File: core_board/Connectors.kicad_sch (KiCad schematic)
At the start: 26 parts, among them J10 Conn_01x04_Pin, J11 Conn_01x04_Pin, J12 Conn_01x04_Pin, J14 Conn_01x04_Pin, J15 Conn_01x04_Pin, J3 Conn_01x04_Pin, J4 Conn_01x04_Pin, J5 Conn_01x04_Pin, J6 Conn_01x04_Pin, J7 Conn_01x02_Pin, J9 Conn_01x02_Pin, Q10 BSS138, Q11 BSS138, Q12 BSS138, Q13 BSS138, Q14 BSS138, Q9 BSS138

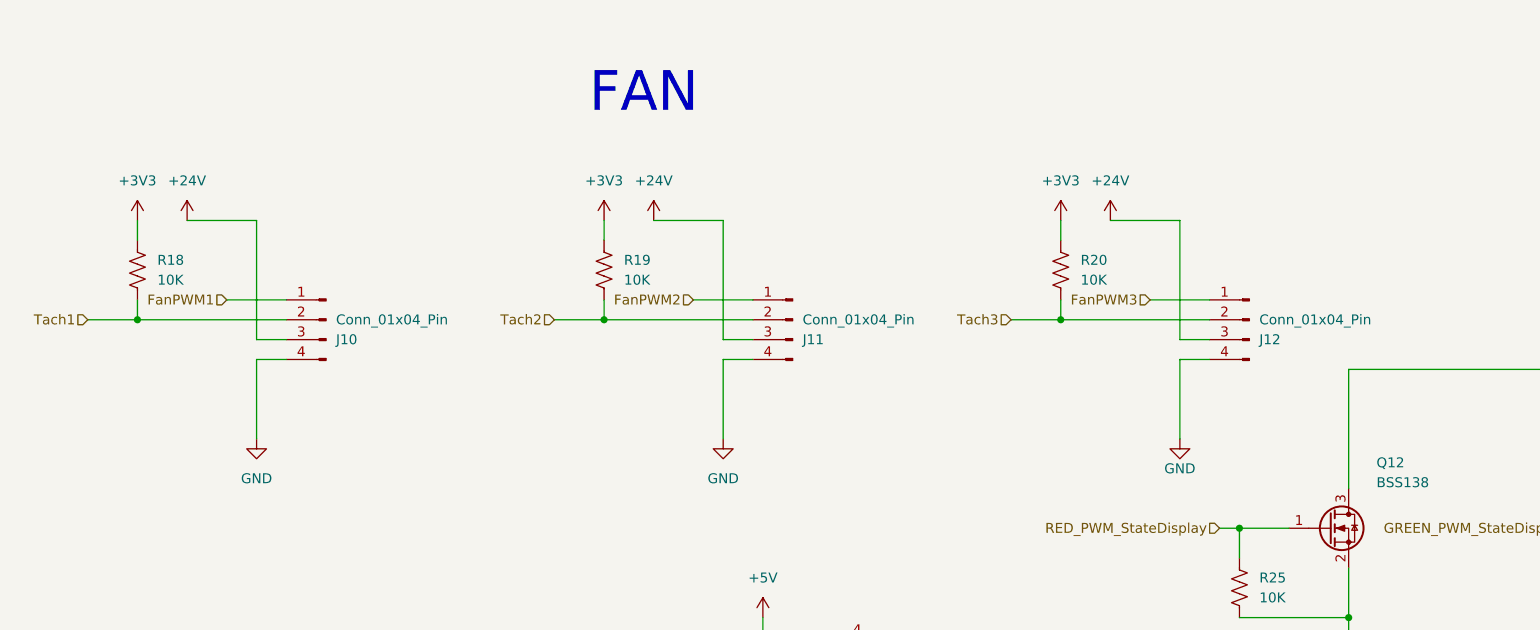
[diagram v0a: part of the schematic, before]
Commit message: Fix fan connectors
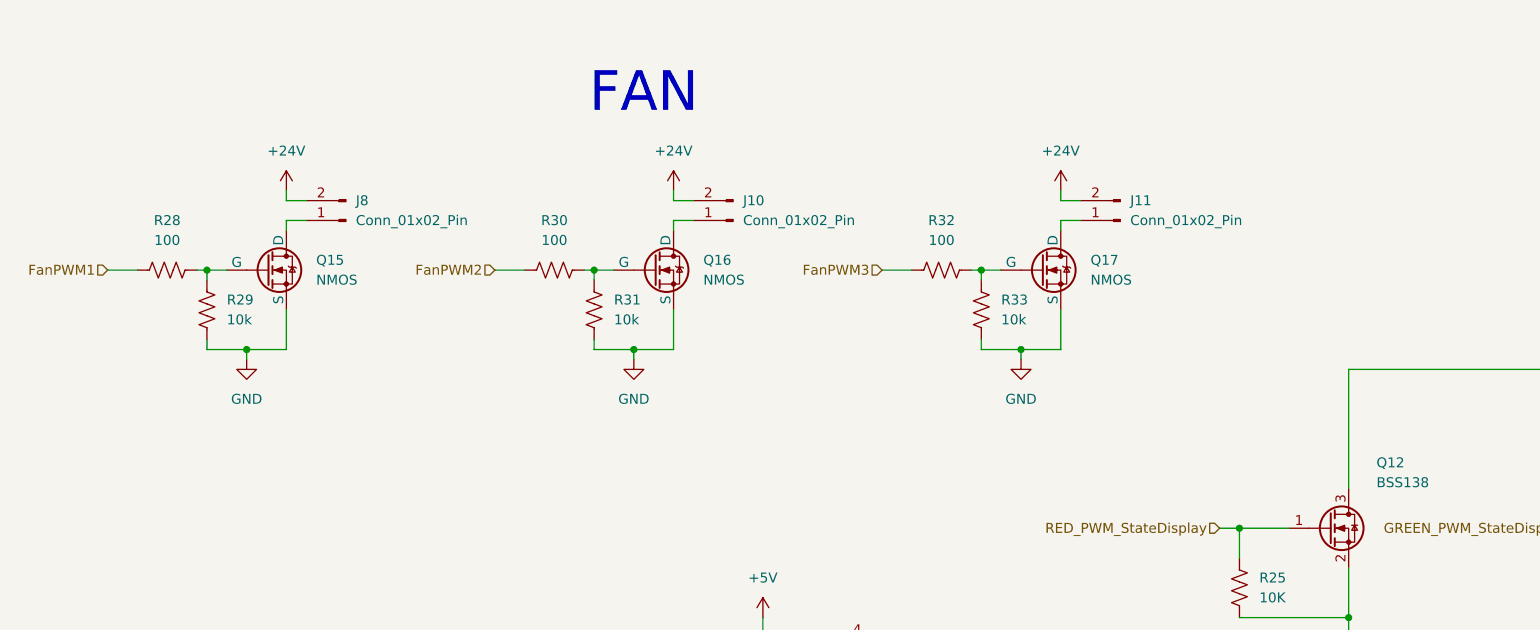
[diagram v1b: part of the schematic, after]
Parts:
- removed J10, J11, J12: Conn_01x04_Pin, Package_DFN_QFN:QFN-20-1EP_5x5mm_P0.65mm_EP3.35x3.35mm, symbol Connector:Conn_01x04_Pin
- removed R18, R19, R20: 10K, Package_DIP:DIP-8_W7.62mm, symbol Device:R_US
- added J10, J11, J8: Conn_01x02_Pin, Converter_DCDC:Converter_DCDC_Cyntec_MUN12AD01-SH, symbol Connector:Conn_01x02_Pin
- added Q15, Q16, Q17: NMOS, Package_DFN_QFN:SiliconLabs_QFN-20-1EP_3x3mm_P0.5mm, symbol Simulation_SPICE:NMOS
- added R28, R30, R32: 100, RF_Module:ESP32-S2-WROVER, symbol Device:R_US
- added R29, R31, R33: 10k, RF_Module:ESP32-S2-WROVER, symbol Device:R_US
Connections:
- net +24V: now also J10.2 (Pin_2), J11.2 (Pin_2), J8.2 (Pin_2)
- net FanPWM1: now also R28.1
- net FanPWM2: now also R30.1
- net FanPWM3: now also R32.1
- net GND: now also Q15.3 (S), Q16.3 (S), Q17.3 (S), R29.1, R31.1, R33.1
- new net: Q16.2 (G), R30.2, R31.2
- new net: J8.1 (Pin_1), Q15.1 (D)
- new net: Q15.2 (G), R28.2, R29.2
- new net: J10.1 (Pin_1), Q16.1 (D)
- new net: J11.1 (Pin_1), Q17.1 (D)
- new net: Q17.2 (G), R32.2, R33.2
